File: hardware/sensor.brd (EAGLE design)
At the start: 100 x 80 mm, 10 parts

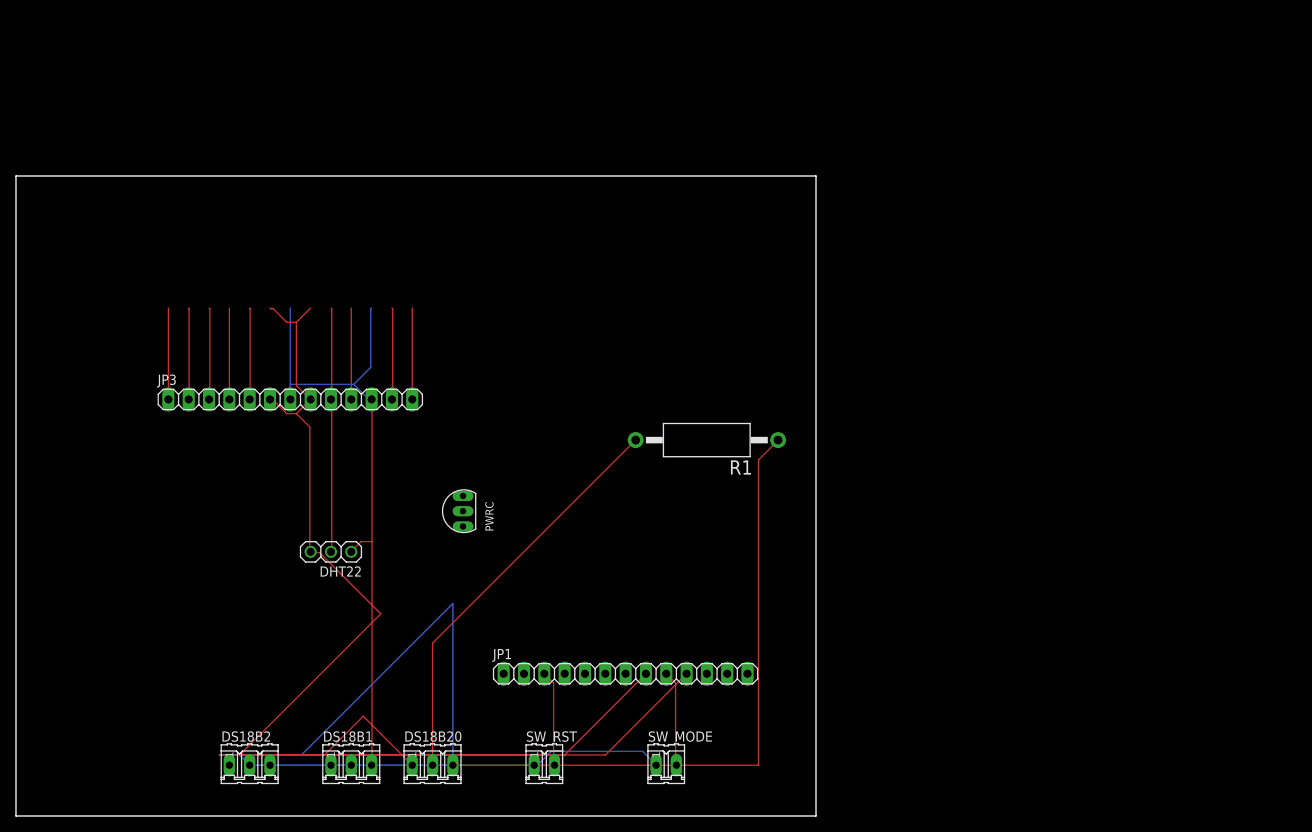
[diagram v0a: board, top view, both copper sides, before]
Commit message: board changes
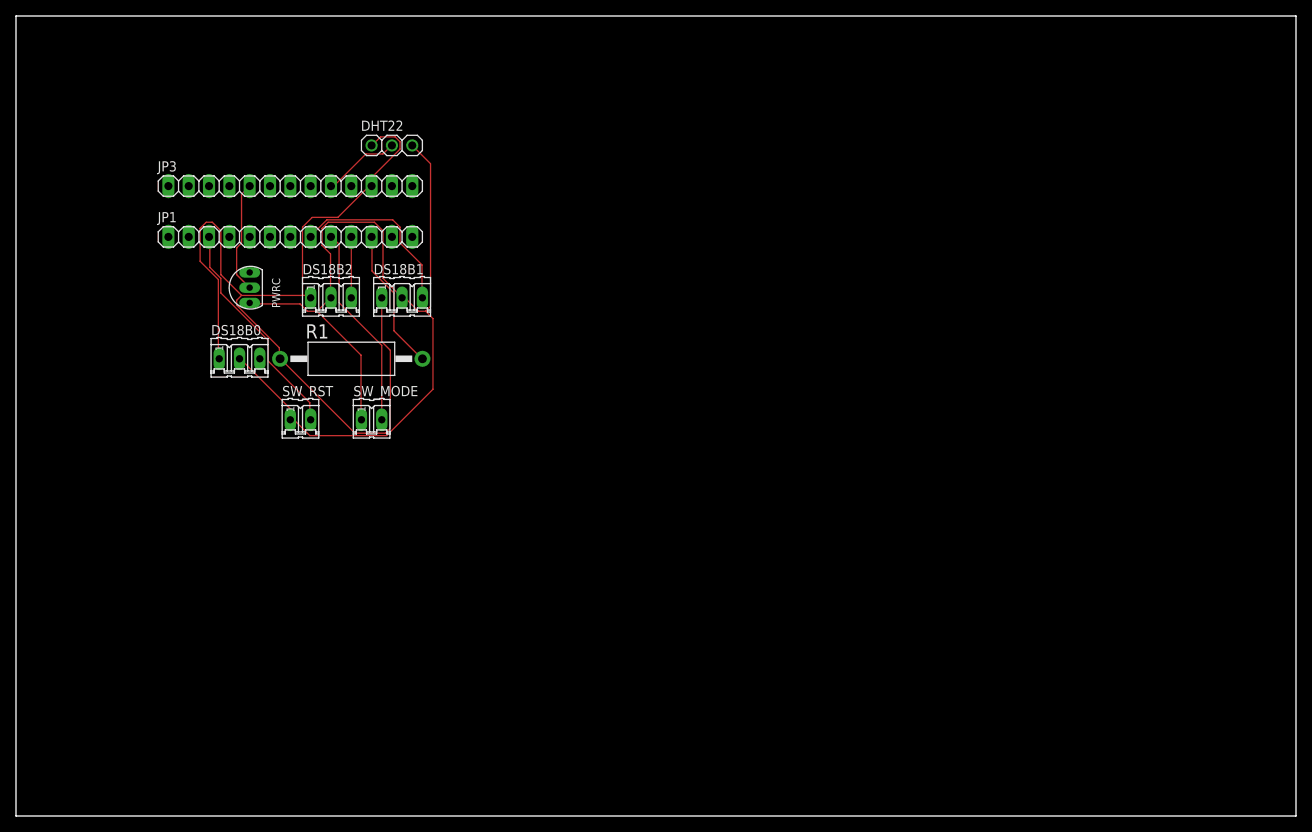
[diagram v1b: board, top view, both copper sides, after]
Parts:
- removed DS18B20: (no value), con-amp-quick:03P
- added DS18B0: (no value), con-amp-quick:03P
- PWRC: value (none) -> 2N7000
- SW_MODE: value (none) -> 1
- SW_RST: value (none) -> 2
- moved JP1 68.8 mm to (34.3, 72.4)
- moved DS18B2 59.3 mm to (39.4, 64.8)
- moved DS18B1 58.8 mm to (48.3, 64.8)
- moved SW_MODE 56.8 mm to (44.5, 49.5)
- moved SW_RST 52.9 mm to (35.6, 49.5)
- moved DHT22 51.4 mm to (47.0, 83.8), turned to 0 degrees
- moved R1 45.6 mm to (41.9, 57.1), turned to 0 degrees
- moved PWRC 38.6 mm to (29.2, 66.0)
- moved JP3 26.7 mm to (34.3, 78.7)
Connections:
- removed net N$1: JP3.1
- removed net N$13: JP3.10
- removed net N$15: JP3.12
- removed net N$16: JP3.13
- removed net N$3: JP1.11
- removed net N$4: JP3.2
- removed net N$6: JP3.3
- removed net N$7: JP3.4
- removed net PGM: JP3.5
- new net EXTGND: PWRC.E
- new net EXT_GND: JP3.8
- new net SENS_EN: JP3.5, PWRC.B
- net 1WIRE: now also DS18B0.3, JP1.11; no longer DS18B20.2
- net 3.3V: now also DS18B0.1, DS18B1.1, DS18B2.1; no longer DS18B20.3, JP3.7
- net AOUT1: now also DS18B2.3
- net AOUT2: now also DS18B1.3
- net GND: now also DS18B0.2, DS18B1.2, DS18B2.2, PWRC.C; no longer DS18B20.1, JP3.6, JP3.8
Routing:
- net 3.3V: track 236.7 -> 114.3 mm
- net AOUT1: track 52.5 -> 7.62 mm
- net GND: track 158.7 -> 121.2 mm
- net 1WIRE: track 51.2 -> 17.9 mm
- net AOUT2: track 49.9 -> 22.7 mm
- net DATA_T: track 30.7 -> 9.72 mm
- net RST: track 12.0 -> 28.2 mm
- net SENS_EN: track 0.00 -> 14.0 mm
- net MODE: track 12.0 -> 25.5 mm
- net N$6: track 11.5 -> 0.00 mm
- net N$15: track 11.5 -> 0.00 mm
- net PGM: track 11.5 -> 0.00 mm
- net N$4: track 11.5 -> 0.00 mm
- net N$7: track 11.4 -> 0.00 mm
- net N$16: track 11.4 -> 0.00 mm
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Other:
- board size 100 x 80 mm -> 160 x 100 mm
- board text added: "DHT22"
- board text added: "DS18B0"
- board text added: "DS18B1"
- board text added: "DS18B2"
- board text added: "JP1"
- board text added: "JP3"
- board text added: "PWRC"
- board text added: "R1"
- board text added: "SW_MODE"
- board text added: "SW_RST"
